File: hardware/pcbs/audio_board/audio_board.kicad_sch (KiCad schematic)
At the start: 16 parts, among them J11 Conn_01x08, J4 NC3MAH, J5 NC3MAH, J6 AudioJack3, J8 I2C

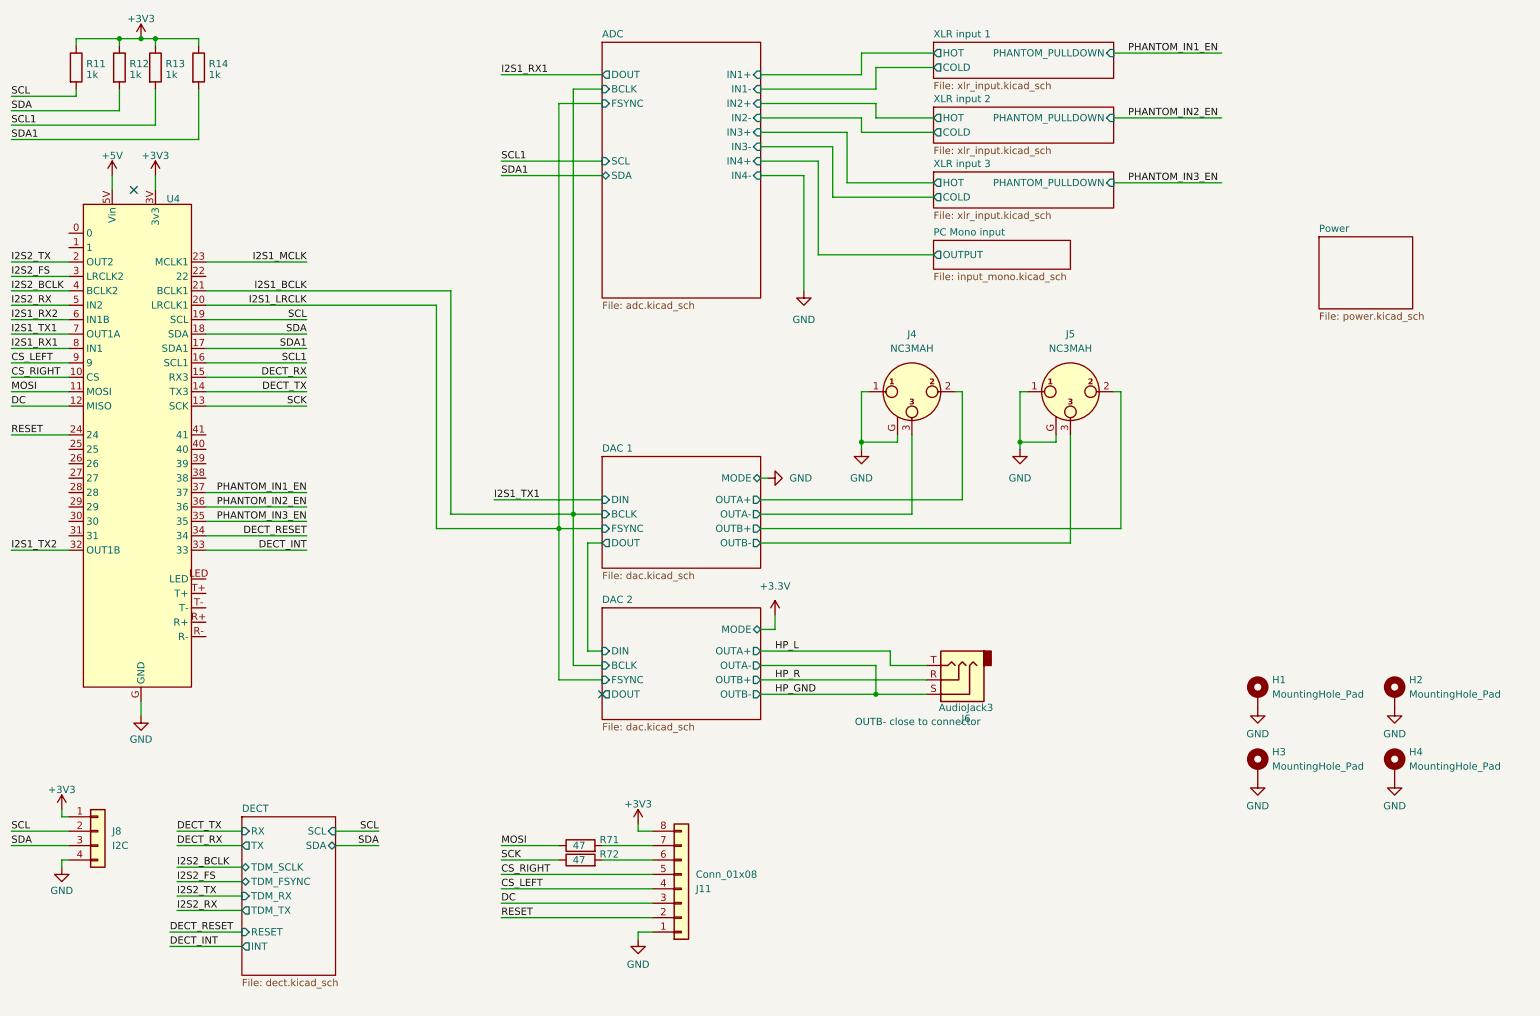
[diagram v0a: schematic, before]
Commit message: fix libraries
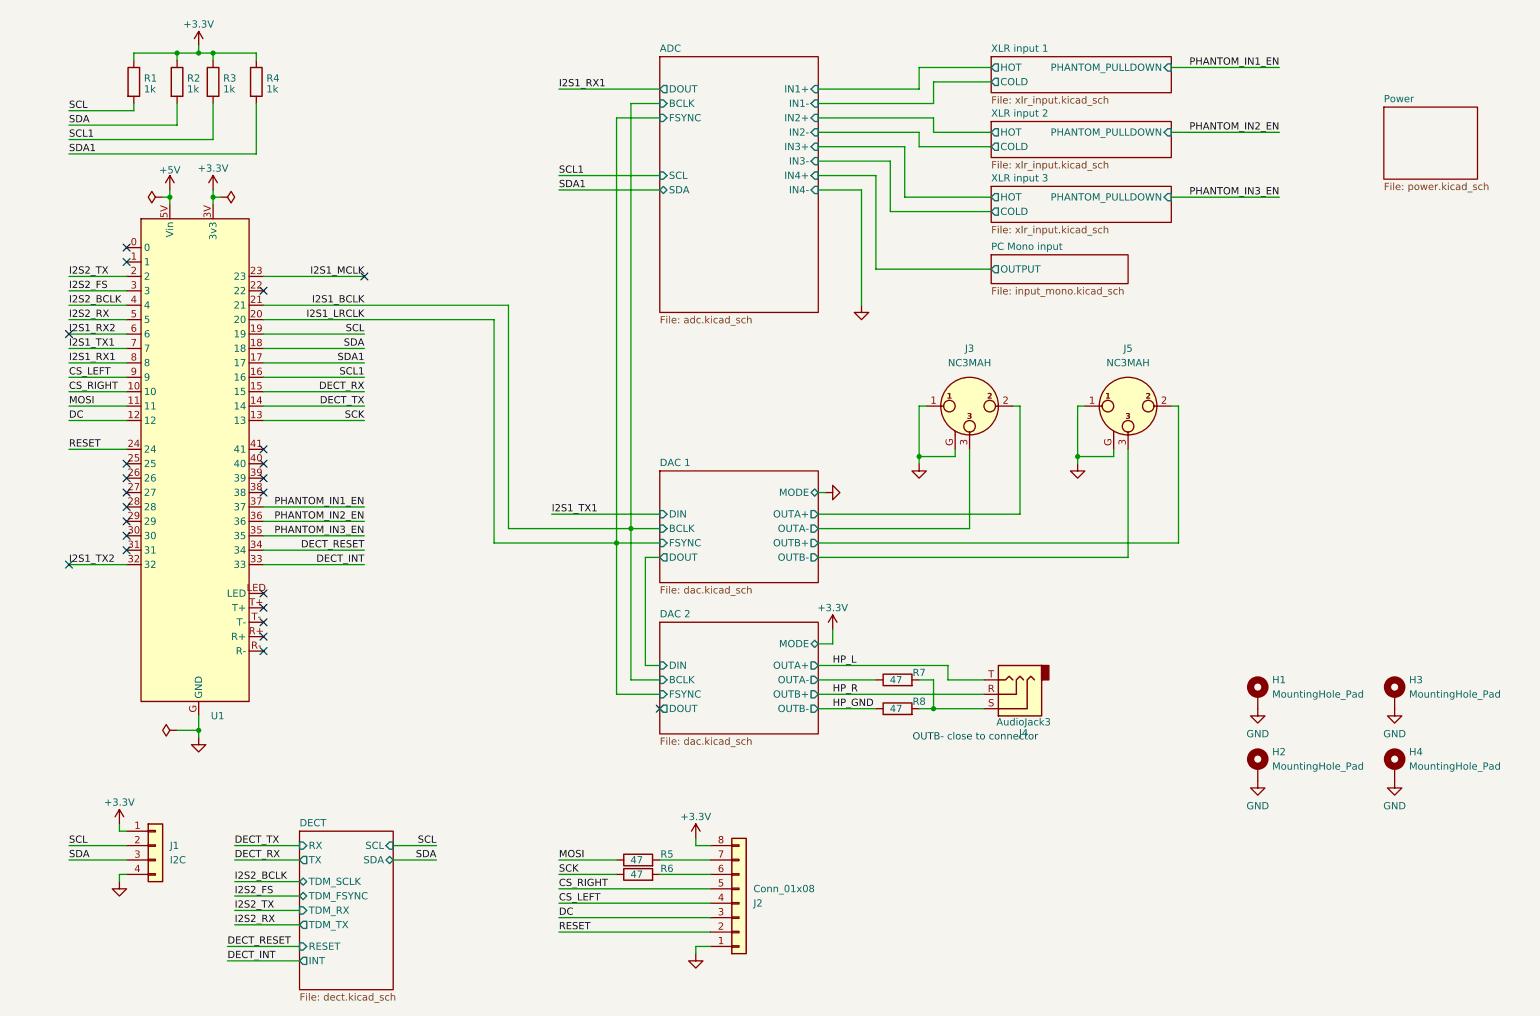
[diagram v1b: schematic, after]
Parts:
- removed U4: ~, Library:Teensy41, symbol Parts:Teensy41
- added R7, R8: 47, Resistor_SMD:R_0805_2012Metric, symbol Device:R
- added U1: ~, extra:Teensy41, symbol extra:Teensy41
- J2: renamed from J11; footprint Library:mta100_01x8_P2.54_647050-8 -> Connector_MTA-100:mta100_01x8_P2.54_647050-8
- renumbered H3 to H2, H2 to H3, J8 to J1, J4 to J3, J6 to J4, R11 to R1, R12 to R2, R13 to R3, R14 to R4, R71 to R5, R72 to R6
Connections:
- net +3V3 is gone; now on net +3.3V: J1.1 (Pin_1), J2.8 (Pin_8), R1.1, R2.1, R3.1, R4.1
- net +3.3V: now also U1.3V (3v3)
- net +5V: now also U1.5V (Vin)
- net CS_LEFT: now also U1.9
- net CS_RIGHT: now also U1.10
- net DC: now also U1.12
- net DECT_INT: now also U1.33
- net DECT_RESET: now also U1.34
- net DECT_RX: now also U1.15
- net DECT_TX: now also U1.14
- net GND: now also U1.G (GND)
- net HP_GND: now also R8.1; no longer J4.S
- net I2S1_BCLK: now also U1.21
- net I2S1_LRCLK: now also U1.20
- net I2S1_MCLK: now also U1.23
- net I2S1_RX1: now also U1.8
- net I2S1_RX2: now also U1.6
- net I2S1_TX1: now also U1.7
- net I2S1_TX2: now also U1.32
- net I2S2_BCLK: now also U1.4
- net I2S2_FS: now also U1.3
- net I2S2_RX: now also U1.5
- net I2S2_TX: now also U1.2
- net MOSI: now also U1.11
- net PHANTOM_IN1_EN: now also U1.37
- net PHANTOM_IN2_EN: now also U1.36
- net PHANTOM_IN3_EN: now also U1.35
- net RESET: now also U1.24
- net SCK: now also U1.13
- net SCL: now also U1.19
- net SCL1: now also U1.16
- net SDA: now also U1.18
- net SDA1: now also U1.17
- new net: J4.S, R7.2, R8.2
- new net DAC 2/OUTA-: R7.1
- no-connect marks 2 -> 23
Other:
- moved on the sheet: J1, J2, J3, J4, J5, R1, R2, R3, R4, R5, R6

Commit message: final touches to libraries
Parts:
- J3, J5: footprint Library:Jack_XLR_Neutrik_NC3MAH_Horizontal -> conn:Jack_XLR_Neutrik_NC3MAH_Horizontal
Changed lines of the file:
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@@
 			)
 		)
-		(property "Footprint" "Library:Jack_XLR_Neutrik_NC3MAH_Horizontal"
+		(property "Footprint" "conn:Jack_XLR_Neutrik_NC3MAH_Horizontal"
 			(at 212.09 85.09 0)
 			(effects
@@
 			)
 		)
-		(property "Footprint" "Library:Jack_XLR_Neutrik_NC3MAH_Horizontal"
+		(property "Footprint" "conn:Jack_XLR_Neutrik_NC3MAH_Horizontal"
 			(at 184.15 85.09 0)
 			(effects
